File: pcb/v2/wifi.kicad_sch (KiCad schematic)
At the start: 19 parts, among them U11 TXS0102DCU, U12 TXS0102DCU, U13 AIC8800

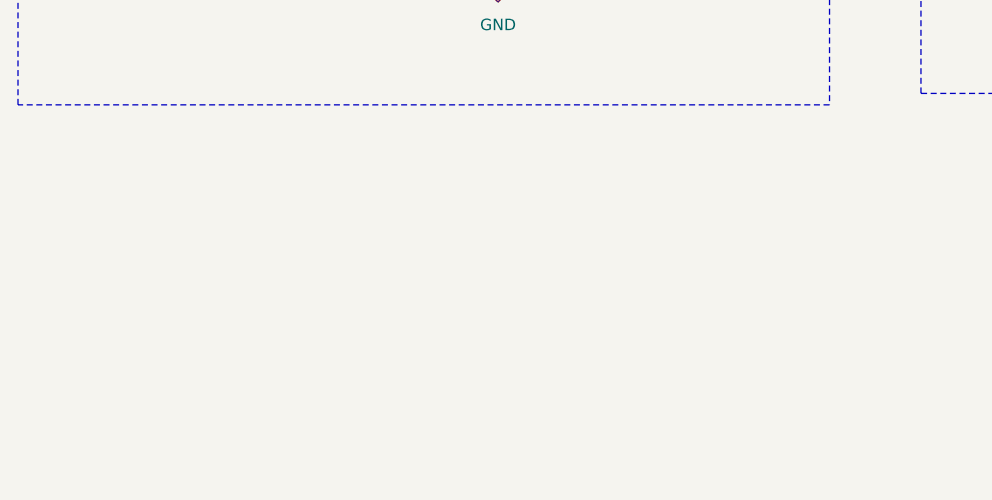
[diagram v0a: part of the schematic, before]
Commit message: up
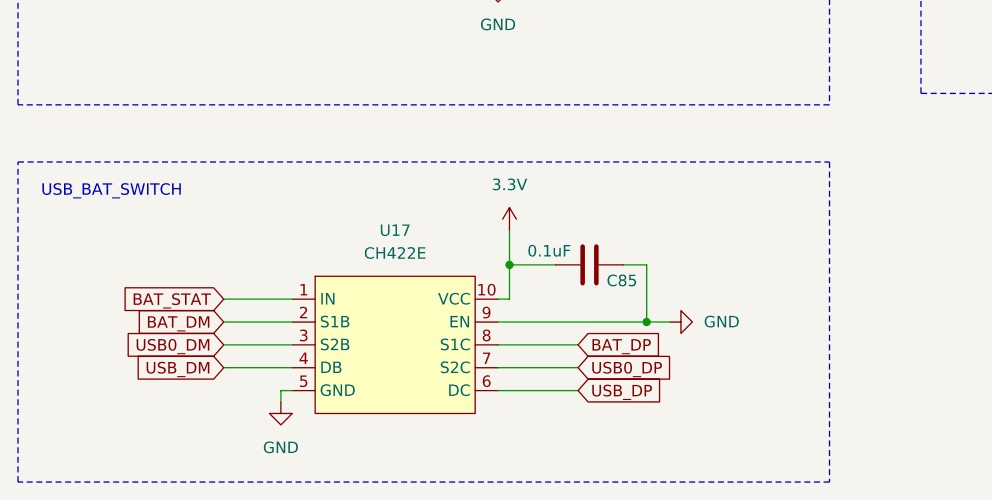
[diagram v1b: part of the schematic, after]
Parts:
- added C85: 0.1uF, Capacitor_SMD:C_0402_1005Metric_Pad0.74x0.62mm_HandSolder, symbol Device:C
- added U17: CH422E, Package_SO:MSOP-10_3x3mm_P0.5mm, symbol coloryr:CH442E
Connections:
- net 3.3V: now also C85.1, U17.10 (VCC)
- net GND: now also C85.2, U17.5 (GND), U17.9 (EN)
- new net BAT_DM: U17.2 (S1B)
- new net BAT_DP: U17.8 (S1C)
- new net BAT_STAT: U17.1 (IN)
- new net USB0_DM: U17.3 (S2B)
- new net USB0_DP: U17.7 (S2C)
- new net USB_DM: U17.4 (DB)
- new net USB_DP: U17.6 (DC)
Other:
- note added: "USB_BAT_SWITCH"

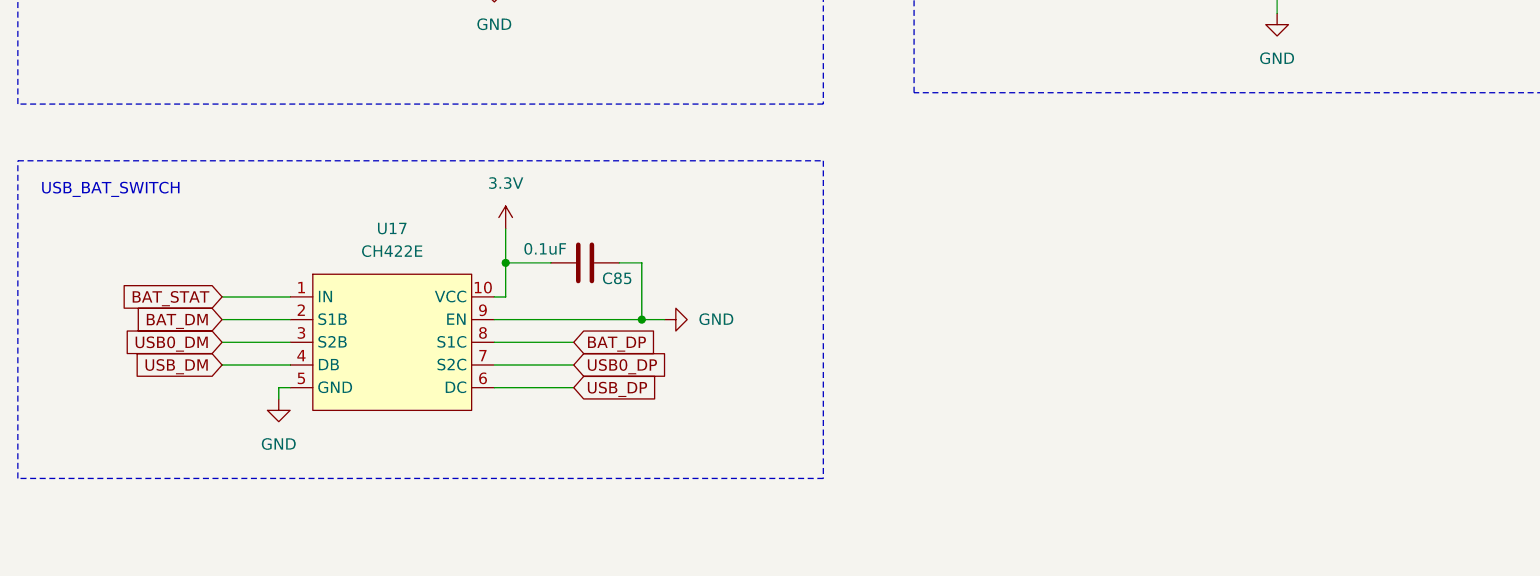
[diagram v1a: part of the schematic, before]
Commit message: up pcb
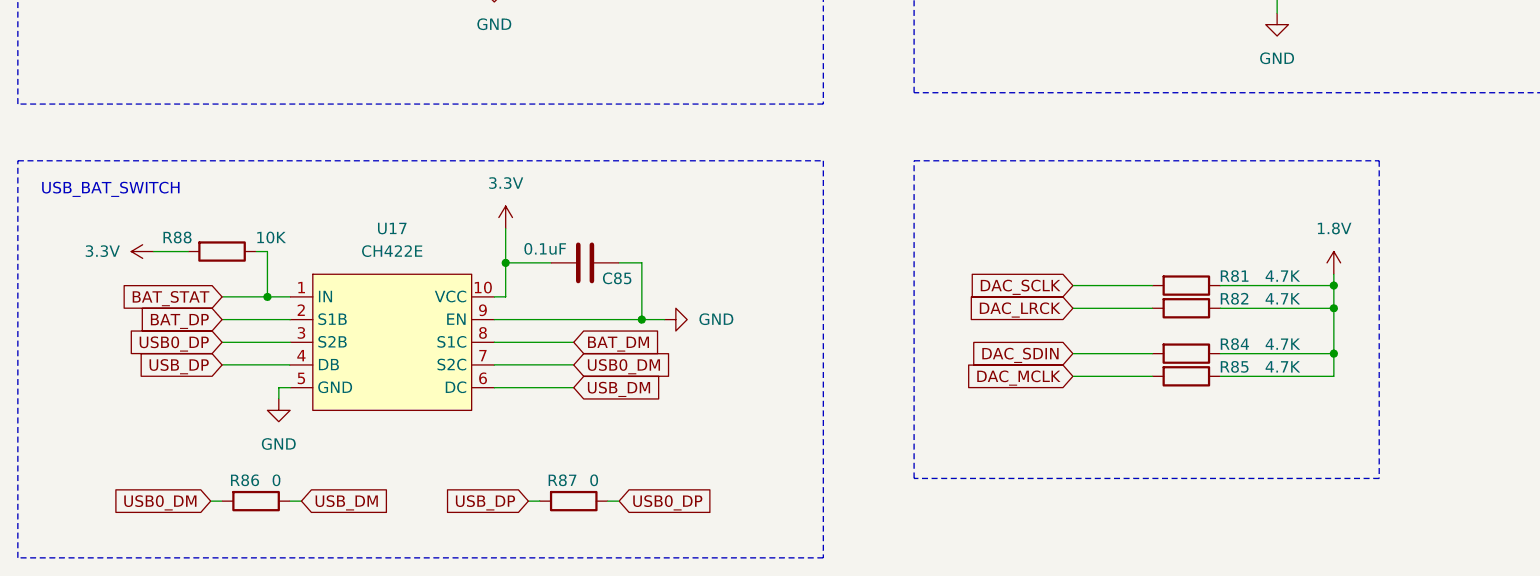
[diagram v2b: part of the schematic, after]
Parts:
- added R81, R82, R84, R85: 4.7K, Capacitor_SMD:C_0402_1005Metric_Pad0.74x0.62mm_HandSolder, symbol Device:R
- added R86, R87: 0, Resistor_SMD:R_0402_1005Metric_Pad0.72x0.64mm_HandSolder, symbol Device:R
- added R88: 10K, Capacitor_SMD:C_0402_1005Metric_Pad0.74x0.62mm_HandSolder, symbol Device:R
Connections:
- net 1.8V: now also R81.1, R82.1, R84.1, R85.1
- net 3.3V: now also R88.2
- net BAT_DM: now also U17.8 (S1C); no longer U17.2 (S1B)
- net BAT_DP: now also U17.2 (S1B); no longer U17.8 (S1C)
- net BAT_STAT: now also R88.1
- net USB0_DM: now also U17.7 (S2C), R86.2; no longer U17.3 (S2B)
- net USB0_DP: now also U17.3 (S2B), R87.1; no longer U17.7 (S2C)
- net USB_DM: now also U17.6 (DC), R86.1; no longer U17.4 (DB)
- net USB_DP: now also U17.4 (DB), R87.2; no longer U17.6 (DC)
- new net DAC_LRCK: R82.2
- new net DAC_MCLK: R85.2
- new net DAC_SCLK: R81.2
- new net DAC_SDIN: R84.2

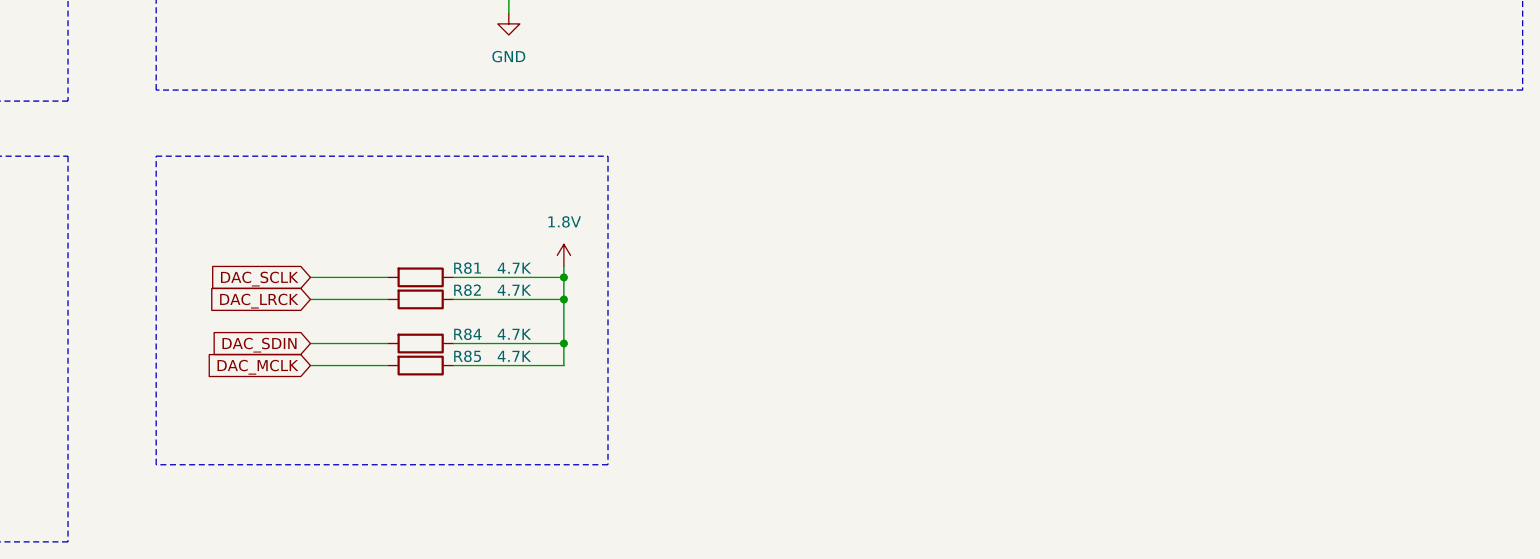
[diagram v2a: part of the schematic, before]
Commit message: up
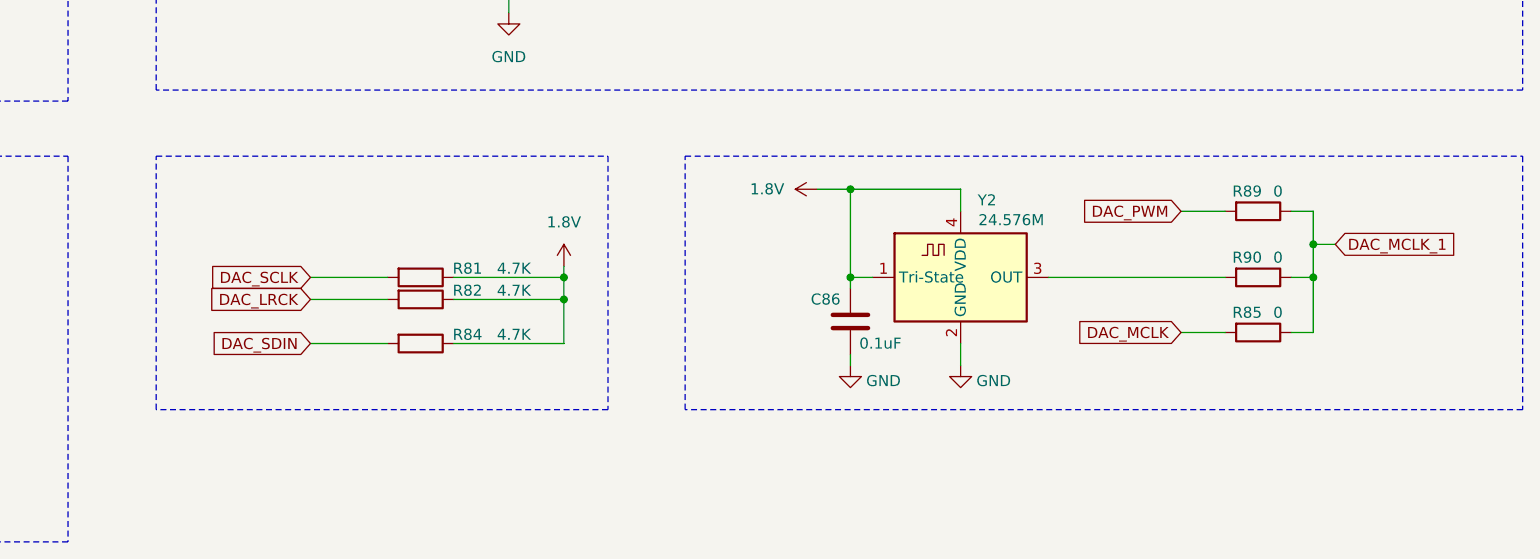
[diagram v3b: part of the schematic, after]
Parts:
- added C86: 0.1uF, Capacitor_SMD:C_0402_1005Metric_Pad0.74x0.62mm_HandSolder, symbol Device:C
- added R89, R90: 0, Resistor_SMD:R_0402_1005Metric_Pad0.72x0.64mm_HandSolder, symbol Device:R
- added Y2: 24.576M, Oscillator:Oscillator_SMD_ECS_2520MV-xxx-xx-4Pin_2.5x2.0mm, symbol Oscillator:ECS-2520MV-xxx-xx
- R85: value 4.7K -> 0; footprint Capacitor_SMD:C_0402_1005Metric_Pad0.74x0.62mm_HandSolder -> Resistor_SMD:R_0402_1005Metric_Pad0.72x0.64mm_HandSolder
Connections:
- net 1.8V: now also C86.1, Y2.1 (Tri-State), Y2.4 (VDD); no longer R85.1
- net GND: now also C86.2, Y2.2 (GND)
- new net: R90.2, Y2.3 (OUT)
- new net DAC_MCLK_1: R85.1, R89.1, R90.1
- new net DAC_PWM: R89.2

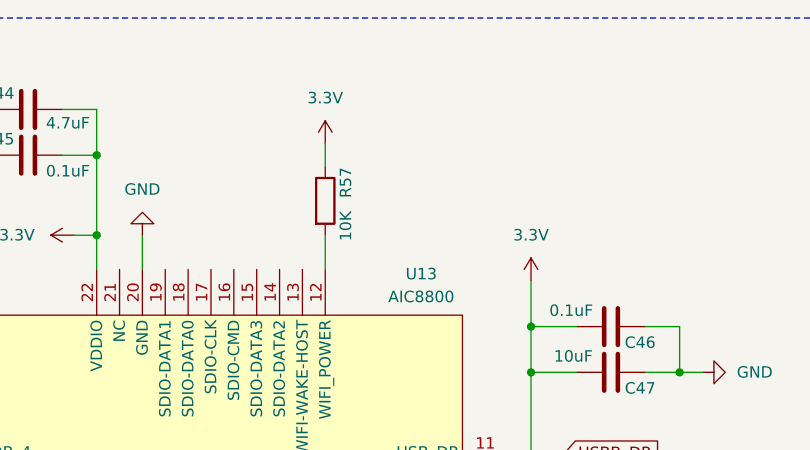
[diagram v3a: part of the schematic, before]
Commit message: up
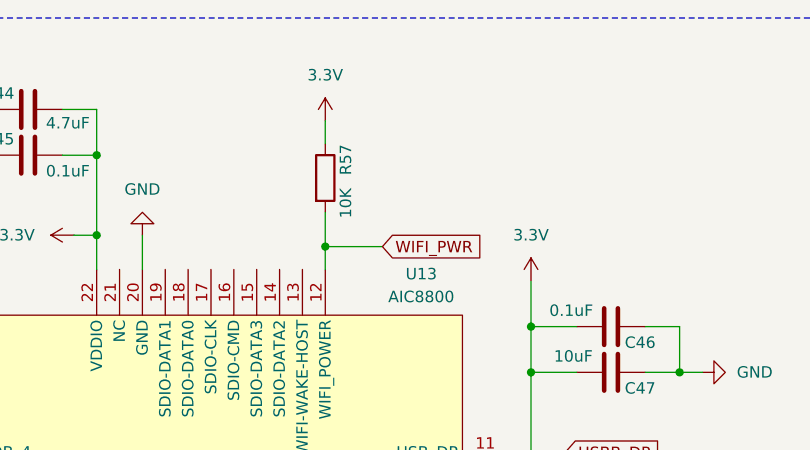
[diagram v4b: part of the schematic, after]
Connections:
- net WIFI_PWR: now reaches R57.2, U13.12 (WIFI_POWER)
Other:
- moved on the sheet: R57
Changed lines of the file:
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@@
 	)
 	(junction
+		(at 181.61 45.72)
+		(diameter 0)
+		(color 0 0 0 0)
+	)
+	(junction
 		(at 156.21 44.45)
 		(diameter 0)
@@
 	(wire
 		(pts
-			(xy 181.61 34.29) (xy 181.61 36.83)
+			(xy 181.61 31.75) (xy 181.61 34.29)
 		)
 		(stroke
@@
 	(wire
 		(pts
+			(xy 181.61 45.72) (xy 187.96 45.72)
+		)
+		(stroke
+			(width 0)
+			(type default)
+		)
+	)
+	(wire
+		(pts
 			(xy 63.5 46.99) (xy 55.88 46.99)
 		)
@@
 	(wire
 		(pts
-			(xy 181.61 44.45) (xy 181.61 48.26)
+			(xy 181.61 41.91) (xy 181.61 45.72)
 		)
 		(stroke
@@
 	(wire
 		(pts
+			(xy 181.61 45.72) (xy 181.61 48.26)
+		)
+		(stroke
+			(width 0)
+			(type default)
+		)
+	)
+	(wire
+		(pts
 			(xy 134.62 93.98) (xy 134.62 95.25)
 		)
@@
 		)
 	)
+	(global_label "WIFI_PWR"
+		(shape input)
+		(at 187.96 45.72 0)
+		(fields_autoplaced yes)
+		(effects
+			(font
+				(size 1.27 1.27)
+			)
+			(justify left)
+		)
+		(property "Intersheetrefs" "${INTERSHEET_REFS}"
+			(at 199.6538 45.72 0)
+			(effects
+				(font
+					(size 1.27 1.27)
+				)
+				(justify left)
+				(hide yes)
+			)
+		)
+	)
 	(global_label "USB0_DM"
 		(shape input)
@@
 	(symbol
 		(lib_id "power:VCC")
-		(at 181.61 34.29 0)
+		(at 181.61 31.75 0)
 		(unit 1)
 		(exclude_from_sim no)
@@
 		(fields_autoplaced yes)
 		(property "Reference" "#PWR094"
-			(at 181.61 38.1 0)
+			(at 181.61 35.56 0)
 			(effects
 				(font
@@
 		)
 		(property "Value" "3.3V"
-			(at 181.61 29.21 0)
+			(at 181.61 26.67 0)
 			(effects
 				(font
@@
 		)
 		(property "Footprint" ""
-			(at 181.61 34.29 0)
+			(at 181.61 31.75 0)
 			(effects
 				(font
@@
 		)
 		(property "Datasheet" ""
-			(at 181.61 34.29 0)
+			(at 181.61 31.75 0)
 			(effects
 				(font
@@
 		)
 		(property "Description" "Power symbol creates a global label with name \"VCC\""
-			(at 181.61 34.29 0)
+			(at 181.61 31.75 0)
 			(effects
 				(font
@@
 	(symbol
 		(lib_id "Device:R")
-		(at 181.61 40.64 0)
+		(at 181.61 38.1 0)
 		(unit 1)
 		(exclude_from_sim no)
@@
 		(dnp no)
 		(property "Reference" "R57"
-			(at 183.896 38.608 90)
+			(at 183.896 36.068 90)
 			(effects
 				(font
@@
 		)
 		(property "Value" "10K"
-			(at 183.896 43.434 90)
+			(at 183.896 40.894 90)
 			(effects
 				(font
@@
 		)
 		(property "Footprint" "Resistor_SMD:R_0402_1005Metric_Pad0.72x0.64mm_HandSolder"
-			(at 179.832 40.64 90)
+			(at 179.832 38.1 90)
 			(effects
 				(font
@@
 		)
 		(property "Datasheet" "~"
-			(at 181.61 40.64 0)
+			(at 181.61 38.1 0)
 			(effects
 				(font
@@
 		)
 		(property "Description" "Resistor"
-			(at 181.61 40.64 0)
+			(at 181.61 38.1 0)
 			(effects
 				(font
